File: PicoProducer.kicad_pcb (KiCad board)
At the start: 2 copper layers, 80 x 61 mm, 37 parts, among them SW1 cherry_mx, SW10 cherry_mx, SW11 cherry_mx, SW12 cherry_mx, SW2 cherry_mx, SW3 cherry_mx, SW4 cherry_mx, SW5 cherry_mx, SW6 cherry_mx, SW7 cherry_mx, SW8 cherry_mx, SW9 cherry_mx, U1 RPI_PICO-SMD

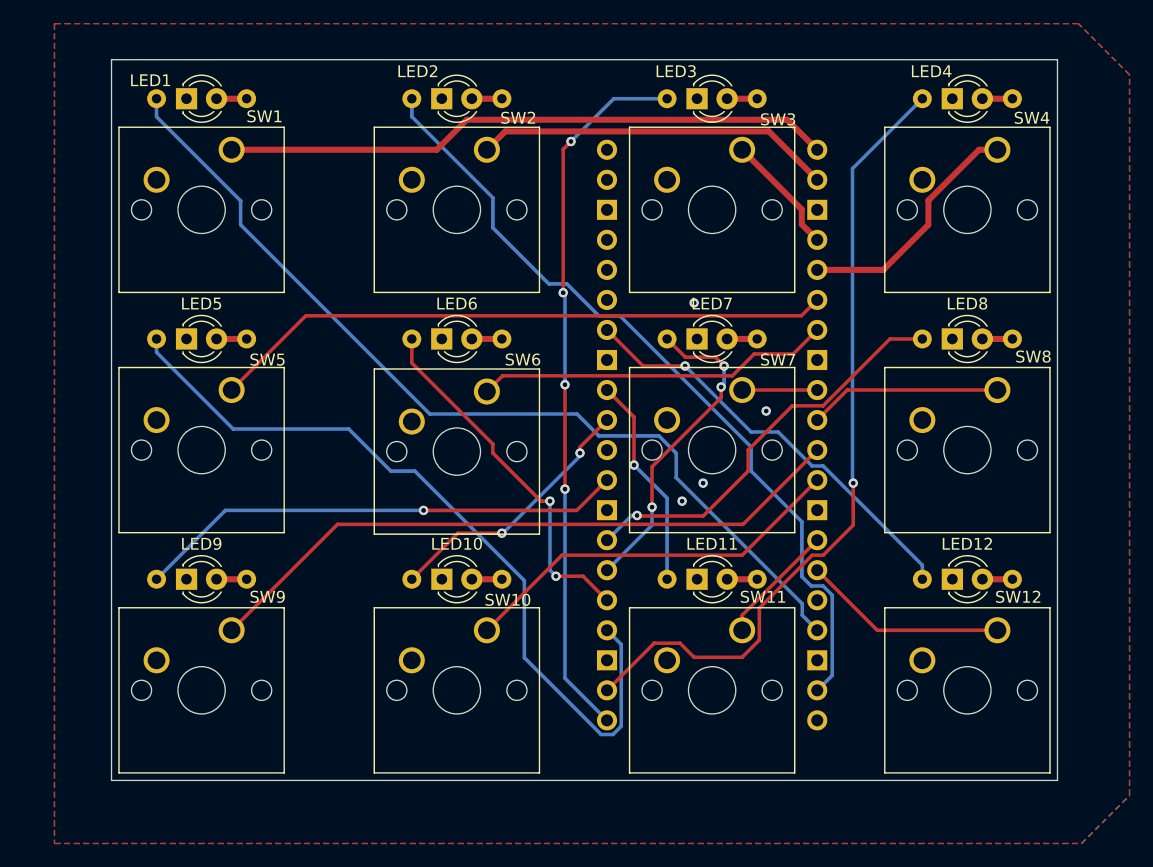
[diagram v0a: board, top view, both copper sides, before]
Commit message: 0.2
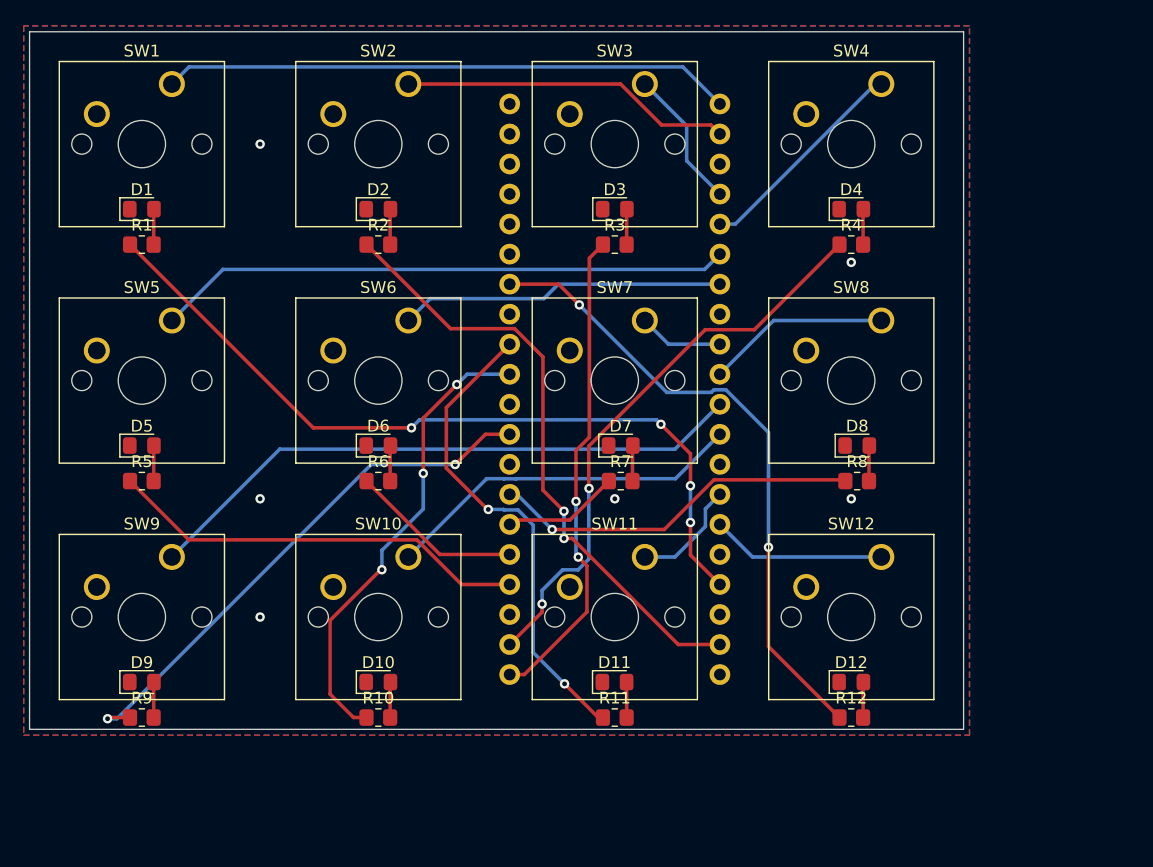
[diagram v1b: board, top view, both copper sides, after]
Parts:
- removed LED1, LED10, LED11, LED12, LED2, LED3, LED4, LED5, LED6, LED7, LED8, LED9: LED, LED_THT:LED_D3.0mm
- added D1: LED, LED_SMD:LED_0805_2012Metric_Pad1.15x1.40mm_HandSolder, F.Cu at (30.0, 35.5)
- added D10: LED, LED_SMD:LED_0805_2012Metric_Pad1.15x1.40mm_HandSolder, F.Cu at (50.0, 75.5)
- added D11: LED, LED_SMD:LED_0805_2012Metric_Pad1.15x1.40mm_HandSolder, F.Cu at (70.0, 75.5)
- added D12: LED, LED_SMD:LED_0805_2012Metric_Pad1.15x1.40mm_HandSolder, F.Cu at (90.0, 75.5)
- added D2: LED, LED_SMD:LED_0805_2012Metric_Pad1.15x1.40mm_HandSolder, F.Cu at (50.0, 35.5)
- added D3: LED, LED_SMD:LED_0805_2012Metric_Pad1.15x1.40mm_HandSolder, F.Cu at (70.0, 35.5)
- added D4: LED, LED_SMD:LED_0805_2012Metric_Pad1.15x1.40mm_HandSolder, F.Cu at (90.0, 35.5)
- added D5: LED, LED_SMD:LED_0805_2012Metric_Pad1.15x1.40mm_HandSolder, F.Cu at (30.0, 55.5)
- added D6: LED, LED_SMD:LED_0805_2012Metric_Pad1.15x1.40mm_HandSolder, F.Cu at (50.0, 55.5)
- added D7: LED, LED_SMD:LED_0805_2012Metric_Pad1.15x1.40mm_HandSolder, F.Cu at (70.5, 55.5)
- added D8: LED, LED_SMD:LED_0805_2012Metric_Pad1.15x1.40mm_HandSolder, F.Cu at (90.5, 55.5)
- added D9: LED, LED_SMD:LED_0805_2012Metric_Pad1.15x1.40mm_HandSolder, F.Cu at (30.0, 75.5)
- R1, R10, R11, R12, R2, R3, R4, R5, R6, R7, R8, R9: footprint Resistor_THT:R_Axial_DIN0207_L6.3mm_D2.5mm_P7.62mm_Horizontal -> Resistor_SMD:R_0805_2012Metric_Pad1.20x1.40mm_HandSolder; moved to F.Cu
- U1: value RPI_PICO-SMD -> Pi Pico; footprint Raspberry Pi:RPi_Pico_SMD_TH -> pi-pico:YD-RP2040
- moved U1 32.9 mm to (70.0, 22.8)
- moved R4 13.7 mm to (90.0, 38.5)
- moved R8 13.2 mm to (90.5, 58.5)
- moved R12 13.2 mm to (90.0, 78.5)
- moved R3 13.1 mm to (70.0, 38.5)
- moved R2 12.7 mm to (50.0, 38.5)
- moved R7 12.6 mm to (70.5, 58.5)
- moved R11 12.5 mm to (70.0, 78.5)
- moved R1 12.4 mm to (30.0, 38.5)
- moved R6 12.3 mm to (50.0, 58.5)
- moved R5 12.1 mm to (30.0, 58.5)
- moved R10 12.0 mm to (50.0, 78.5)
- moved R9 11.8 mm to (30.0, 78.5)
- moved SW12 11.6 mm to (92.5, 64.9)
- moved SW8 11.4 mm to (92.5, 44.9)
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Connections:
- net Net-(U1-GPIO0) renamed /GP0
- net Net-(U1-GPIO1) renamed /GP1
- net Net-(U1-GPIO10) renamed /GP10
- net Net-(U1-GPIO11) renamed /GP11
- net Net-(U1-GPIO13) renamed /GP13
- net Net-(U1-GPIO14) renamed /GP14
- net Net-(U1-GPIO16) renamed /GP16
- net Net-(U1-GPIO17) renamed /GP17
- net Net-(U1-GPIO18) renamed /GP18
- net Net-(U1-GPIO19) renamed /GP19
- net Net-(U1-GPIO2) renamed /GP2
- net Net-(U1-GPIO20) renamed /GP20
- net Net-(U1-GPIO21) renamed /GP21
- net Net-(U1-GPIO22) renamed /GP22
- net Net-(U1-GPIO26_ADC0) renamed /GP26
- net Net-(U1-GPIO27_ADC1) renamed /GP27
- net Net-(U1-GPIO28_ADC2) renamed /GP28
- net Net-(U1-GPIO3) renamed /GP3
- net Net-(U1-GPIO4) renamed /GP4
- net Net-(U1-GPIO5) renamed /GP5
- net Net-(U1-GPIO6) renamed /GP6
- net Net-(U1-GPIO7) renamed /GP7
- net Net-(U1-GPIO8) renamed /GP8
- net Net-(U1-GPIO9) renamed /GP9
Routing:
- net /GP18: track 66.5 -> 35.7 mm
- net /GP27: track 18.1 -> 41.0 mm, vias 1 -> 2
- net /GP16: track 60.4 -> 41.1 mm, vias 4 -> 2
- net /GP17: track 67.7 -> 48.6 mm, vias 1 -> 2
- net /GP28: track 36.1 -> 53.9 mm, vias 1 -> 2
- net /GP20: track 27.1 -> 9.91 mm, vias 3 -> 0
- net /GP26: track 22.5 -> 39.4 mm, vias 2 -> 3
- net /GP19: track 30.7 -> 14.7 mm, vias 2 -> 0
- net /GP14: track 67.8 -> 51.8 mm, vias 0 -> 2
- net /GP13: track 78.4 -> 67.4 mm, vias 0 -> 4
- net /GP22: track 41.6 -> 45.9 mm, vias 1 -> 2
- net /GP8: track 55.8 -> 51.7 mm
- net /GP4: track 52.7 -> 48.7 mm
- net /GP21: track 34.8 -> 31.4 mm
- net /GP0: track 51.6 -> 48.2 mm
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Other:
- board size 80 x 61 mm -> 79 x 59 mm
- board text added: "@qdon.space@blue_on Pico Producer Remix revised 2024 Sep."
- board text removed: "@qdon.space@blue_on @pete_codes"
- board text removed: "pico producer fork by Blue_ON, 2023 Dec. based on Pico Producer V1.0 - © Pete Gallagher 2021"
